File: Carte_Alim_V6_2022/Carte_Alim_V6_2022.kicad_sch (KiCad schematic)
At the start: 56 parts, among them J1 BAT_IN, J10 12VC, J11 12VC, J12 12VC, J13 12VP, J14 12VP, J15 12VP, J16 12VP, J17 12VP, J18 12VP, J19 5VC, J2 BAT_IN, J20 5V_CAN, J21 5VC, J22 5V_CAN, J23 5VC, J24 5V_CAN, J25 5VC, J26 5V_CAN, J27 5VP, J28 5VP, J29 5VP, J3 MOT_OUT, J30 5VP, J31 5VP, J32 5VP, J4 MOT_OUT, J5 MOT_OUT, J6 MOT_OUT, J7 12VC, J8 12VC, J9 12VC

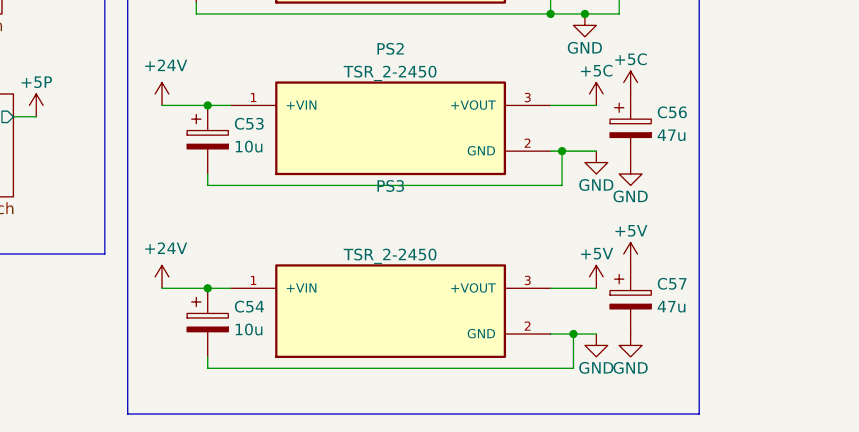
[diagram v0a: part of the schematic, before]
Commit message: modif carte alim
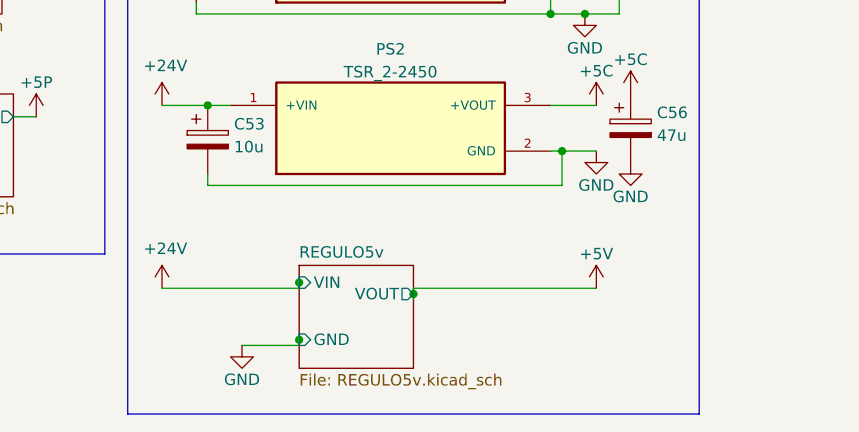
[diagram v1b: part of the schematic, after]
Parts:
- removed C54: 10u, Capacitor_THT:CP_Radial_D4.0mm_P2.00mm, symbol Device:C_Polarized
- removed C57: 47u, Capacitor_THT:CP_Radial_D4.0mm_P2.00mm, symbol Device:C_Polarized
- removed PS3: TSR_2-2450, AREA_lib_composant:CONV_TSR_2-2450, symbol AREA_composant:TSR_2-2450
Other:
- added sheet REGULO5v (REGULO5v.kicad_sch)
